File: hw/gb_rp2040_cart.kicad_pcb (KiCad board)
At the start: 2 copper layers, 51.4 x 60.5 mm, 59 parts, among them J1 GameBoy_Cartridge, J2 USB, J3 USB_BOOT, J4 Expansion, Q1 PMH550UPE, Q2 RU1J002YN, U1 CLXC8T245QRHLRQ1, U2 CLXC8T245QRHLRQ1, U3 CLXC8T245QRHLRQ1, U4 TXU0104, U5 W25Q128JVSIM, U6 RP2040, U7 NCP167, U8 RV-3129-C3, U9 PCA9536D, Y1 12M

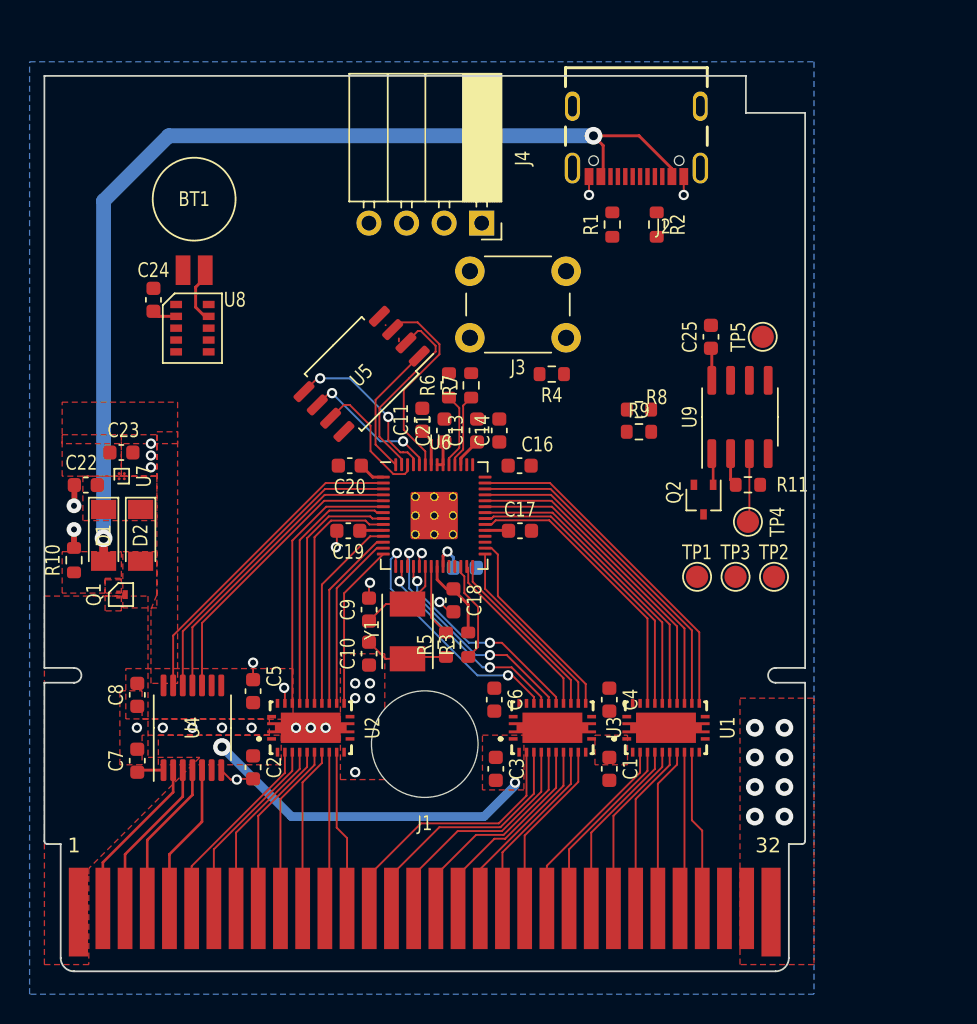
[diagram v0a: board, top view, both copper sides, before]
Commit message: hw: complete 2-layer PCB
Signed-off-by: Mahyar Koshkouei <mk@deltabeard.com>
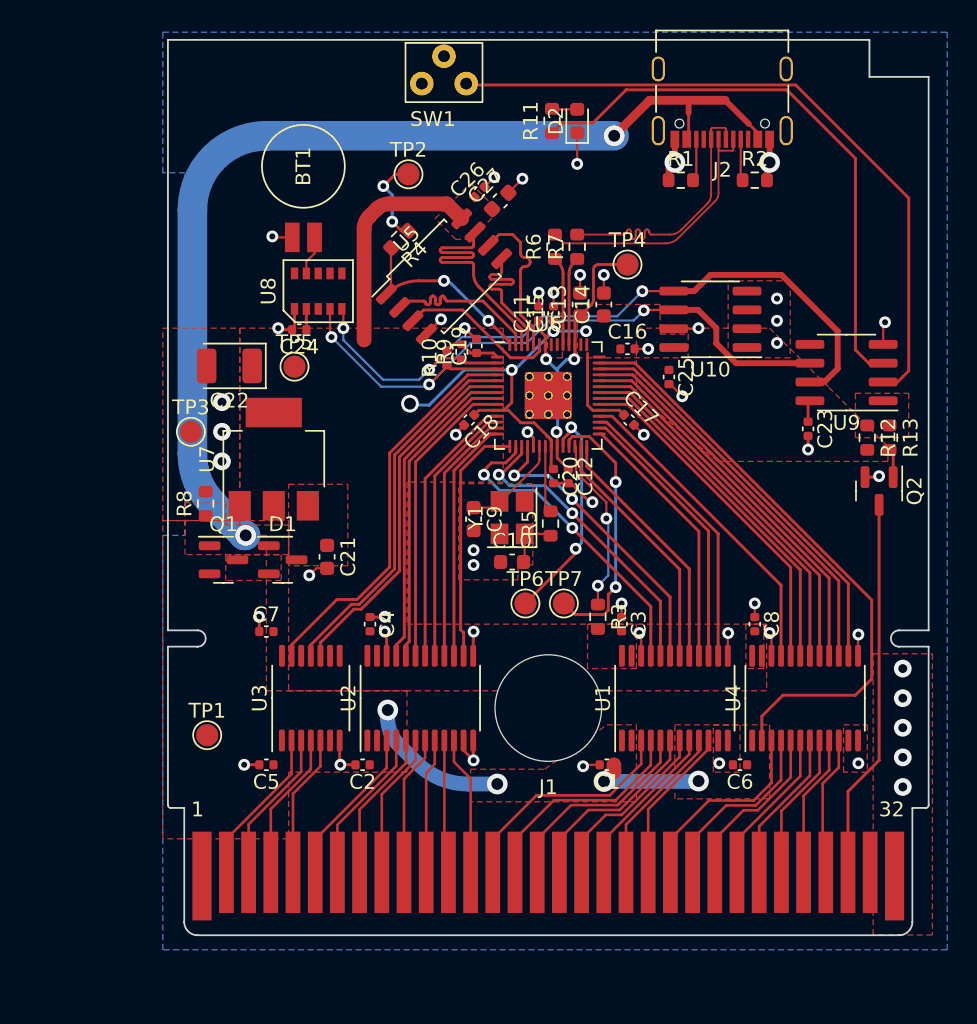
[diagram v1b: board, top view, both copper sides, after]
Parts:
- removed J3: USB_BOOT, Button_Switch_THT:SW_PUSH_6mm
- removed J4: Expansion, Connector_PinSocket_2.54mm:PinSocket_1x04_P2.54mm_Horizontal
- added C15: 100n, Capacitor_SMD:C_0402_1005Metric, F.Cu at (84.4, 56.0)
- added C26: 100n, Capacitor_SMD:C_0402_1005Metric, F.Cu at (79.4, 47.8)
- added C27: 2.2u, Capacitor_SMD:C_0603_1608Metric, F.Cu at (80.8, 48.4)
- added R12: 100k, Resistor_SMD:R_0603_1608Metric, F.Cu at (105.6, 64.4)
- added R13: 330R, Resistor_SMD:R_0603_1608Metric, F.Cu at (107.1, 64.4)
- added SW1: SW_SPST, Project_Specific:Push_Button-Horizontal-TC-1109DE-C-J, F.Cu at (77.0, 38.6)
- added TP6: SWCLK, TestPoint:TestPoint_Pad_D1.5mm, F.Cu at (82.5, 75.6)
- added TP7: SWDIO, TestPoint:TestPoint_Pad_D1.5mm, F.Cu at (85.1, 75.6)
- added U10: MB85RC256VPNF-G-JNERE1, Package_SO:SOIC-8_3.9x4.9mm_P1.27mm, F.Cu at (95.0, 56.4)
- BT1: value MS621FE -> Battery_Cell
- C1, C11, C16, C17, C18, C19, C2, C20, C24, C25, C3, C4, C5, C6, C7, C8: footprint Capacitor_SMD:C_0603_1608Metric -> Capacitor_SMD:C_0402_1005Metric
- C10, C9: value 27p -> 30p
- C12: footprint Capacitor_SMD:C_0603_1608Metric -> Capacitor_SMD:C_0402_1005Metric; moved to F.Cu
- C21: value 100n -> 2.2u
- C22: value 2.2u -> 100u; footprint Capacitor_SMD:C_0603_1608Metric -> Capacitor_Tantalum_SMD:CP_EIA-3528-15_AVX-H
- C23: value 2.2u -> 100n; footprint Capacitor_SMD:C_0603_1608Metric -> Capacitor_SMD:C_0402_1005Metric
- D1: value FDLL4148 -> D_Dual_CommonCathode_AAK_Split; footprint Diode_SMD:D_MiniMELF -> Package_TO_SOT_SMD:SOT-23
- D2: value FDLL4148 -> LED; footprint Diode_SMD:D_MiniMELF -> LED_SMD:LED_0603_1608Metric
- J2: value USB -> USB_C_Receptacle_USB2.0; footprint Project_Specific:GCT_USB4105-GF-A -> Connector_USB:USB_C_Receptacle_Palconn_UTC16-G
- Q1: value PMH550UPE -> SI2301CDS-T1-GE3; footprint Project_Specific:DFN0606-3 -> Package_TO_SOT_SMD:SOT-23
- Q2: value RU1J002YN -> N-Channel; footprint Package_TO_SOT_SMD:SOT-323_SC-70 -> Package_TO_SOT_SMD:SOT-23
- R10: value 100k -> 4k7; footprint Resistor_SMD:R_0603_1608Metric -> Resistor_SMD:R_0402_1005Metric
- R11: value 100k -> 330R
- R8: value 5k1 -> 100k
- R9: value 5k1 -> 4k7; footprint Resistor_SMD:R_0603_1608Metric -> Resistor_SMD:R_0402_1005Metric
- TP1: value SWCLK -> TestPoint
- TP2: value SWDIO -> TestPoint
- TP3: value GND -> TestPoint
- TP4: value IO2 -> TestPoint
- TP5: value IO3 -> TestPoint
- U1, U2: value CLXC8T245QRHLRQ1 -> SN74LVC8T245PW; footprint Project_Specific:CLXC8T245QRHLRQ1 -> Package_SO:TSSOP-24_4.4x7.8mm_P0.65mm
- U3: value CLXC8T245QRHLRQ1 -> TXU0104; footprint Project_Specific:CLXC8T245QRHLRQ1 -> Package_SO:TSSOP-14_4.4x5mm_P0.65mm
- U4: value TXU0104 -> SN74LVC8T245PW; footprint Package_SO:TSSOP-14_4.4x5mm_P0.65mm -> Package_SO:TSSOP-24_4.4x7.8mm_P0.65mm
- U5: value W25Q128JVSIM -> W25Q128JVSIQ
- U7: value NCP167 -> AMS1117-3.3; footprint Project_Specific:WLCSP-4-0.64x0.64mm_P0.35mm -> Package_TO_SOT_SMD:SOT-223-3_TabPin2
- U8: footprint Project_Specific:DFN-10-2.5x2.7mm-P0.8 -> Project_Specific:SOIC-10_RV-3129-C3
- Y1: value 12M -> Crystal_GND24; footprint Crystal:Crystal_SMD_TXC_7A-2Pin_5x3.2mm -> Crystal:Crystal_SMD_3225-4Pin_3.2x2.5mm
- moved C23 46.4 mm to (101.6, 63.8), turned to -90 degrees
- moved C8 42.0 mm to (98.0, 77.0), turned to -90 degrees
- moved U4 41.4 mm to (101.4, 82.0)
- moved D2 40.7 mm to (86.0, 43.0), turned to 90 degrees
- moved TP3 38.1 mm to (59.9, 64.0)
- moved TP2 36.7 mm to (74.6, 46.6)
- moved TP1 34.8 mm to (61.0, 84.5)
- moved TP5 31.7 mm to (66.9, 59.6), turned to 0 degrees
- moved R8 30.0 mm to (60.9, 68.8), turned to 90 degrees
- moved R10 28.7 mm to (77.2, 59.0)
- moved R11 27.9 mm to (84.3, 43.0), turned to 90 degrees
- moved TP4 19.2 mm to (89.4, 52.7), turned to 0 degrees
- moved C6 17.2 mm to (97.0, 86.5), turned to 180 degrees
- moved C4 17.0 mm to (72.0, 77.0)
- moved U3 16.4 mm to (68.0, 82.0)
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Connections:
- net /Peripherals/VBAT renamed Net-(BT1-Pad1)
- C21 pad 1: +3V3 -> +5V
- C22 pad 1: +5V -> +3V3
- C24 pad 1: GND -> +3V3
- C24 pad 2: +3V3 -> GND
- C3 pad 1: GB_5V -> GND
- C3 pad 2: GND -> +3V3
- C5 pad 1: GND -> GB_5V
- C5 pad 2: +3V3 -> GND
- C6 pad 1: GND -> GB_5V
- C6 pad 2: +3V3 -> GND
- C7 pad 1: GB_5V -> GND
- C7 pad 2: GND -> +3V3
- D1 pad 1: +5V -> VBUS
- D1 pad 2: VBUS -> Net-(D1-Pad2)
- D2 pad 1: +5V -> GND
- J2 pad A6: USB_DP -> USB_DN
- J2 pad A7: USB_DN -> USB_DP
- J2 pad B6: USB_DP -> USB_DN
- J2 pad B7: USB_DN -> USB_DP
- Q1 pad 3: Net-(D2-Pad2) -> Net-(D1-Pad2)
- Q2 pad 1: /Peripherals/RESET_GB -> Net-(Q2-Pad1)
- R10 pad 1: VBUS -> I^{2}C_{SCL}
- R10 pad 2: GND -> +3V3
- R11 pad 1: GND -> Net-(R11-Pad1)
- R11 pad 2: GB_5V -> Net-(D2-Pad2)
- R8 pad 1: +3V3 -> VBUS
- R8 pad 2: I2C_SDA -> GND
- R9 pad 1: +3V3 -> I^{2}C_{SDA}
- R9 pad 2: I2C_SCL -> +3V3
- TP1 pad 1: /RP2040/SWCLK -> GB_5V
- TP2 pad 1: /RP2040/SWDIO -> /RP2040/USB_BOOT
- TP4 pad 1: Net-(TP4-Pad1) -> +1V1
- TP5 pad 1: Net-(TP5-Pad1) -> +3V3
- U1 pad 10: /D7 -> /A15
- U1 pad 14: 3V3_D7 -> 3V3_A15
- U1 pad 15: 3V3_D6 -> 3V3_A14
- U1 pad 16: 3V3_D5 -> 3V3_A13
- U1 pad 17: 3V3_D4 -> 3V3_A12
- U1 pad 18: 3V3_D3 -> 3V3_A11
- U1 pad 19: 3V3_D2 -> 3V3_A10
- U1 pad 2: ~{RD} -> GB_5V
- U1 pad 20: 3V3_D1 -> 3V3_A9
- U1 pad 21: 3V3_D0 -> 3V3_A8
- U1 pad 3: /D0 -> /A8
- U1 pad 4: /D1 -> /A9
- U1 pad 5: /D2 -> /A10
- U1 pad 6: /D3 -> /A11
- U1 pad 7: /D4 -> /A12
- U1 pad 8: /D5 -> /A13
- U1 pad 9: /D6 -> /A14
- U3 pad 10: /A15 -> ~{CS}_3V3
- U3 pad 11: GND -> ~{RD}_3V3
- U3 pad 12: GND -> ~{WR}_3V3
- U3 pad 13: GND -> PHI_3V3
- U3 pad 14: 3V3_A15 -> +3V3
- U3 pad 2: GB_5V -> PHI
- U3 pad 3: /A8 -> ~{WR}
- U3 pad 4: /A9 -> ~{RD}
- U3 pad 5: /A10 -> ~{CS}
- U3 pad 6: /A11 -> (no net)
- U3 pad 7: /A12 -> GND
- U3 pad 8: /A13 -> +3V3
- U3 pad 9: /A14 -> (no net)
- U4 pad 10: ~{CS}_3V3 -> /D7
- U4 pad 11: ~{RD}_3V3 -> GND
- U4 pad 12: ~{WR}_3V3 -> GND
- U4 pad 13: PHI_3V3 -> GND
- U4 pad 14: +3V3 -> 3V3_D7
- U4 pad 2: PHI -> DATA_DIR
- U4 pad 3: ~{WR} -> /D0
- U4 pad 4: ~{RD} -> /D1
- U4 pad 5: ~{CS} -> /D2
- U4 pad 6: (no net) -> /D3
- U4 pad 7: GND -> /D4
- U4 pad 8: +3V3 -> /D5
- U4 pad 9: (no net) -> /D6
- U6 pad 11: 3V3_A4 -> 3V3_A3
- U6 pad 12: 3V3_A5 -> 3V3_A4
- U6 pad 13: 3V3_A6 -> 3V3_A5
- U6 pad 14: 3V3_A7 -> 3V3_A6
- U6 pad 15: 3V3_A8 -> 3V3_A7
- U6 pad 16: 3V3_A9 -> 3V3_A8
- U6 pad 17: 3V3_A10 -> 3V3_A9
- U6 pad 18: 3V3_A11 -> 3V3_A10
- U6 pad 2: PHI_3V3 -> I^{2}C_{SDA}
- U6 pad 27: 3V3_A12 -> 3V3_A11
- U6 pad 28: 3V3_A13 -> 3V3_A12
- U6 pad 29: 3V3_A14 -> 3V3_A13
- U6 pad 3: ~{WR}_3V3 -> I^{2}C_{SCL}
- U6 pad 30: 3V3_A15 -> 3V3_A14
- U6 pad 31: I2C_SDA -> 3V3_A15
- U6 pad 32: I2C_SCL -> 3V3_D0
- U6 pad 34: 3V3_D0 -> 3V3_D1
- U6 pad 35: 3V3_D1 -> 3V3_D2
- U6 pad 36: 3V3_D2 -> 3V3_D3
- U6 pad 37: 3V3_D3 -> 3V3_D4
- U6 pad 38: 3V3_D4 -> 3V3_D5
- U6 pad 39: 3V3_D5 -> 3V3_D6
- U6 pad 4: ~{RD}_3V3 -> PHI_3V3
- U6 pad 40: 3V3_D6 -> 3V3_D7
- U6 pad 41: 3V3_D7 -> DATA_DIR
- U6 pad 5: ~{CS}_3V3 -> ~{RD}_3V3
- U6 pad 6: 3V3_A0 -> ~{CS}_3V3
- U6 pad 7: 3V3_A1 -> 3V3_A0
- U6 pad 8: 3V3_A2 -> 3V3_A1
- U6 pad 9: 3V3_A3 -> 3V3_A2
- U8 pad 10: (no net) -> unconnected-(U8-Pad10)
- U8 pad 4: I2C_SCL -> I^{2}C_{SCL}
- U8 pad 5: I2C_SDA -> I^{2}C_{SDA}
- U9 pad 1: /Peripherals/RESET_GB -> GB_RESET
- U9 pad 2: GB_5V -> Net-(SW1-Pad1)
- U9 pad 3: Net-(TP4-Pad1) -> Net-(R11-Pad1)
- U9 pad 5: Net-(TP5-Pad1) -> unconnected-(U9-Pad5)
- U9 pad 6: I2C_SCL -> I^{2}C_{SCL}
- U9 pad 7: I2C_SDA -> I^{2}C_{SDA}
- Y1 pad 2: Net-(C9-Pad1) -> GND
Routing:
- net I^{2}C_{SDA}: track 0.00 -> 50.7 mm, vias 0 -> 3
- net Net-(SW1-Pad1): track 0.00 -> 46.7 mm
- net I^{2}C_{SCL}: track 0.00 -> 45.1 mm, vias 0 -> 3
- net GND: track 14.2 -> 56.2 mm, vias 35 -> 53
- net DATA_DIR: track 0.00 -> 40.5 mm
- net Net-(R11-Pad1): track 0.00 -> 38.8 mm
- net +3V3: track 16.5 -> 53.9 mm, vias 0 -> 4
- net ~{RES}: track 0.00 -> 25.6 mm
- net ~{WR}_3V3: track 21.2 -> 0.00 mm
- net USB_DN: track 0.00 -> 18.9 mm
- net USB_DP: track 0.00 -> 18.2 mm
- net /RP2040/SWDIO: track 0.00 -> 18.0 mm, vias 0 -> 2
- net /RP2040/SWCLK: track 0.00 -> 15.3 mm, vias 0 -> 2
- net +1V1: track 6.90 -> 21.5 mm, vias 1 -> 3
- net GB_5V: track 26.9 -> 17.9 mm, vias 2 -> 4
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- added copper zone on F.Cu, net GB_RESET
- added copper zone on F.Cu, net Net-(D1-Pad2)
- removed copper zone on F.Cu, net Net-(D2-Pad2)
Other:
- outline, holes or cut-outs redrawn
